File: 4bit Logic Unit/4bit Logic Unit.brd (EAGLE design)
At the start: 161.3 x 110.2 mm, 91 parts

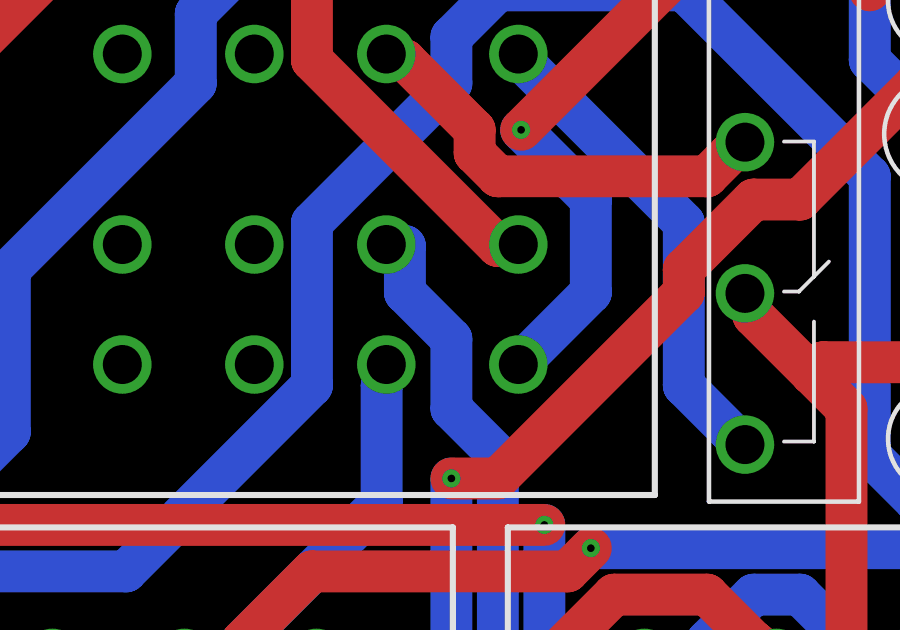
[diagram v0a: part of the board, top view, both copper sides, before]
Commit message: Minor formatting changes
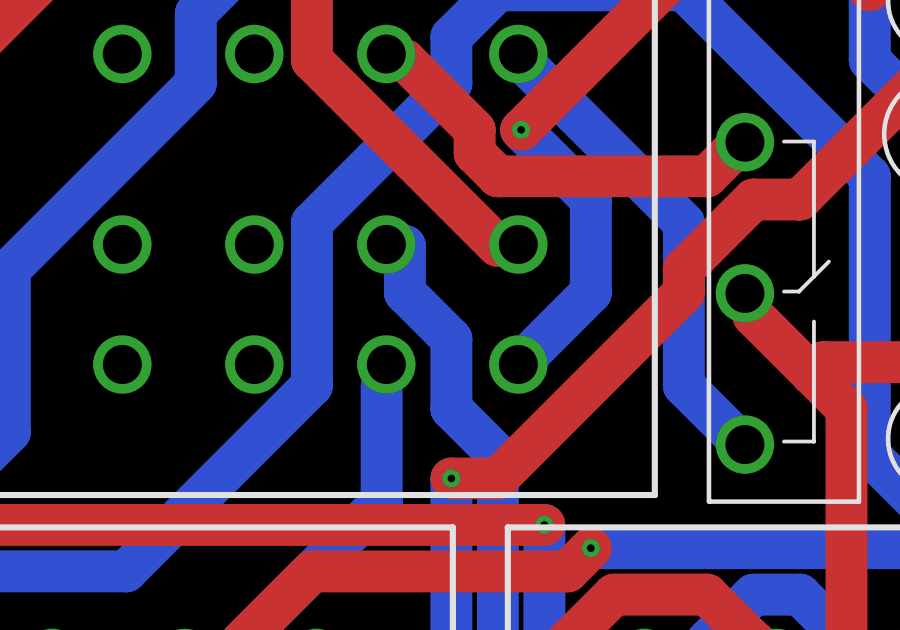
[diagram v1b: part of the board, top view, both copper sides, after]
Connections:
- net N$19: now also 2-4_DECODER:K2.44; no longer 2-4_DECODER:K2.32
- net N$22: now also 2-4_DECODER:K2.32; no longer 2-4_DECODER:K2.44
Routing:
- net N$19: track 111.0 -> 110.3 mm
- net N$22: track 233.7 -> 233.0 mm
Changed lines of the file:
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@@
 <?xml version="1.0" encoding="utf-8"?>
 <!DOCTYPE eagle SYSTEM "eagle.dtd">
-<eagle version="8.3.2">
+<eagle version="8.4.3">
 <drawing>
 <settings>
@@
 <param name="dpMaxLengthDifference" value="10mm"/>
 <param name="dpGapFactor" value="2.5"/>
-<param name="checkGrid" value="0"/>
 <param name="checkAngle" value="0"/>
 <param name="checkFont" value="1"/>
 <param name="checkRestrict" value="1"/>
+<param name="checkStop" value="0"/>
 <param name="useDiameter" value="13"/>
 <param name="maxErrors" value="50"/>
@@
 <contactref element="LOGIC8-1:ENABLE_NOT:K1" pad="A2"/>
 <contactref element="LOGIC8-1:ENABLE_NOT:D1" pad="C"/>
-<contactref element="2-4_DECODER:K2" pad="32"/>
 <wire x1="127.8255" y1="43.3832" x2="127.8255" y2="34.8615" width="1.397" layer="1"/>
 <wire x1="127.8255" y1="34.8615" x2="128.143" y2="34.544" width="1.397" layer="1"/>
@@
 <wire x1="124.7267" y1="46.482" x2="116.9797" y2="46.482" width="1.397" layer="16"/>
 <wire x1="127.0508" y1="44.1579" x2="124.7267" y2="46.482" width="1.397" layer="16"/>
-<wire x1="70.4977" y1="69.723" x2="70.653" y2="70.422" width="1.397" layer="16"/>
 <wire x1="127.0508" y1="44.1579" x2="127.512" y2="43.942" width="1.397" layer="16"/>
 <via x="80.5688" y="41.0591" extent="1-16" drill="0.254"/>
@@
 <via x="106.9086" y="37.9603" extent="1-16" drill="0.254"/>
 <via x="106.9086" y="41.0591" extent="1-16" drill="0.254"/>
+<contactref element="2-4_DECODER:K2" pad="44"/>
+<wire x1="70.4977" y1="69.723" x2="75.053" y2="74.422" width="0" layer="19" extent="16-16"/>
 </signal>
 <signal name="N$20">
@@
 <contactref element="LOGIC8-1:ENABLE_XOR:K1" pad="A2"/>
 <contactref element="LOGIC8-1:ENABLE_XOR:D1" pad="C"/>
-<contactref element="2-4_DECODER:K2" pad="44"/>
 <wire x1="106.1339" y1="8.5217" x2="106.1339" y2="1.5494" width="1.397" layer="1"/>
 <wire x1="104.5845" y1="10.0711" x2="106.1339" y2="8.5217" width="1.397" layer="1"/>
@@
 <wire x1="119.3038" y1="8.5217" x2="135.5725" y2="8.5217" width="1.397" layer="16"/>
 <wire x1="106.1339" y1="8.5217" x2="119.3038" y2="8.5217" width="1.397" layer="1"/>
-<wire x1="74.3712" y1="74.3712" x2="75.053" y2="74.422" width="1.397" layer="1"/>
 <via x="72.8218" y="97.6122" extent="1-16" drill="0.254"/>
 <via x="127.0508" y="104.5845" extent="1-16" drill="0.254"/>
@@
 <via x="144.0942" y="17.0434" extent="1-16" drill="0.254"/>
 <via x="119.3038" y="8.5217" extent="1-16" drill="0.254"/>
+<contactref element="2-4_DECODER:K2" pad="32"/>
+<wire x1="74.3712" y1="74.3712" x2="70.653" y2="70.422" width="0" layer="19" extent="1-1"/>
 </signal>
 <signal name="LOGIC8-1:NOT3">
